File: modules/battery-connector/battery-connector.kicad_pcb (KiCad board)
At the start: 2 copper layers, 15 x 12.7 mm, 2 parts, among them J1 691210910002

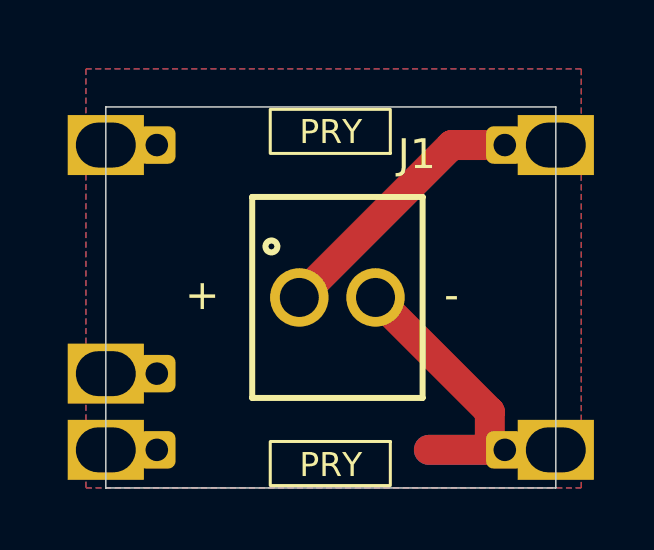
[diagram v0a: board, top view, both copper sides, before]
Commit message: Updating all modules
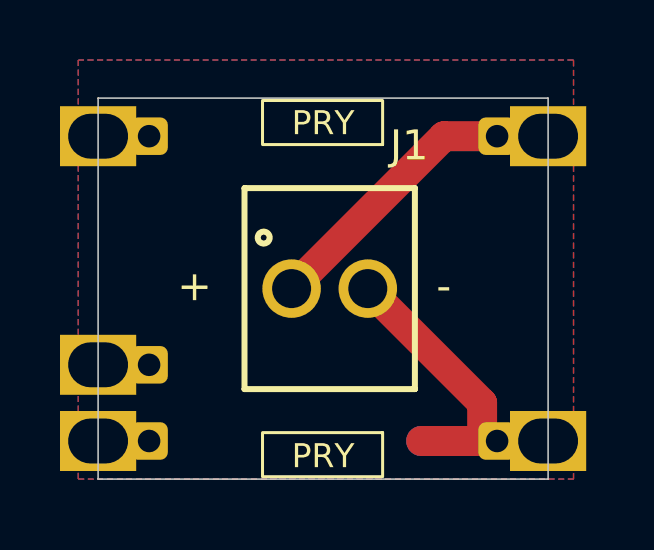
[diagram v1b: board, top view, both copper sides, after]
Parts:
- moved J1 0.39 mm to (67.8, 61.3)
- moved M1 0.39 mm to (67.6, 61.3)
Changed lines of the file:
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@@
 	(footprint "MegaCastle:691210910002"
 		(layer "F.Cu")
-		(at 68.032 61.58)
+		(at 67.775 61.285)
 		(descr "<b>WR-TBL Serie 2109 - 2.54 mm Horiz. Entry<br></b>Max Height =8.5mm , Pitch 2.54mm , 2 Pins")
 		(property "Reference" "J1"
@@
 	(footprint "MegaCastle:MegaCastle2x5-Module-I15.0x7.9-M8CC-SPAREPAD"
 		(layer "B.Cu")
-		(at 67.812 61.58 180)
+		(at 67.555 61.285 180)
 		(property "Reference" "M1"
 			(at -2.948 -5.65 0)
@@
 			(polygon
 				(pts
-					(xy 69.796241 56.778592) (xy 69.796241 55.31) (xy 65.792484 55.31) (xy 65.792484 56.778592)
+					(xy 69.539241 56.483592) (xy 69.539241 55.015) (xy 65.535484 55.015) (xy 65.535484 56.483592)
 				)
 			)
@@
 			(polygon
 				(pts
-					(xy 69.796241 66.381408) (xy 69.796241 67.85) (xy 65.792484 67.85) (xy 65.792484 66.381408)
+					(xy 69.539241 66.086408) (xy 69.539241 67.555) (xy 65.535484 67.555) (xy 65.535484 66.086408)
 				)
 			)
@@
 			(polygon
 				(pts
-					(xy 75.312 55.23) (xy 75.312 57.63) (xy 60.312 57.63) (xy 60.312 55.23)
+					(xy 75.055 54.935) (xy 75.055 57.335) (xy 60.055 57.335) (xy 60.055 54.935)
 				)
 			)
@@
 			(polygon
 				(pts
-					(xy 75.312 67.93) (xy 75.312 65.53) (xy 60.312 65.53) (xy 60.312 67.93)
+					(xy 75.055 67.635) (xy 75.055 65.235) (xy 60.055 65.235) (xy 60.055 67.635)
 				)
 			)
@@
 	)
 	(gr_text "-"
-		(at 71.588 62.088 0)
+		(at 71.331 61.793 0)
 		(layer "F.SilkS")
 		(effects
@@
 	)
 	(gr_text "+"
-		(at 62.952 62.088 0)
+		(at 62.695 61.793 0)
 		(layer "F.SilkS")
 		(effects
@@
 	)
 	(gr_text "R20250405"
-		(at 65.0856 58.3542 90)
+		(at 64.8286 58.0592 90)
 		(layer "B.SilkS")
 		(effects
@@
 	)
 	(segment
-		(start 73.112 56.5)
-		(end 71.842 56.5)
+		(start 72.855 56.205)
+		(end 71.585 56.205)
 		(width 1)
 		(layer "F.Cu")
@@
 	)
 	(segment
-		(start 71.842 56.5)
-		(end 66.762 61.58)
+		(start 71.585 56.205)
+		(end 66.505 61.285)
 		(width 1)
 		(layer "F.Cu")
@@
 	)
 	(segment
-		(start 73.112 66.66)
-		(end 73.112 65.39)
+		(start 72.855 66.365)
+		(end 72.855 65.095)
 		(width 1)
 		(layer "F.Cu")
@@
 	)
 	(segment
-		(start 73.112 65.39)
-		(end 69.302 61.58)
+		(start 72.855 65.095)
+		(end 69.045 61.285)
 		(width 1)
 		(layer "F.Cu")
@@
 	)
 	(segment
-		(start 73.112 66.66)
-		(end 71.08 66.66)
+		(start 72.855 66.365)
+		(end 70.823 66.365)
 		(width 1)
 		(layer "F.Cu")
@@
 	)
 	(segment
-		(start 73.112 66.66)
-		(end 71.08 66.66)
+		(start 72.855 66.365)
+		(end 70.823 66.365)
 		(width 1)
 		(layer "B.Cu")
@@
 		(polygon
 			(pts
-				(xy 59.65 53.96) (xy 59.65 67.93) (xy 76.16 67.93) (xy 76.16 53.96)
-			)
-		)
+				(xy 59.393 53.665) (xy 59.393 67.635) (xy 75.903 67.635) (xy 75.903 53.665)
+			)
+		)
